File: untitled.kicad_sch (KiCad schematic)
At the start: 11 parts, among them U5 LM76005

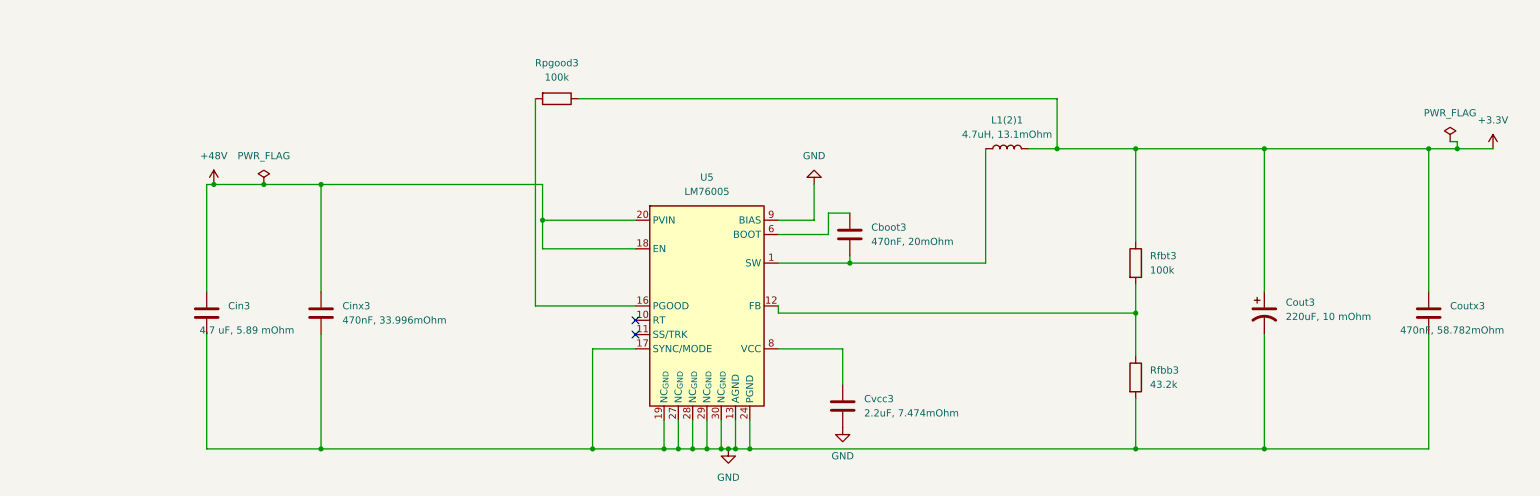
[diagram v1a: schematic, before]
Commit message: Fixed Schematics with more cost effective IC's
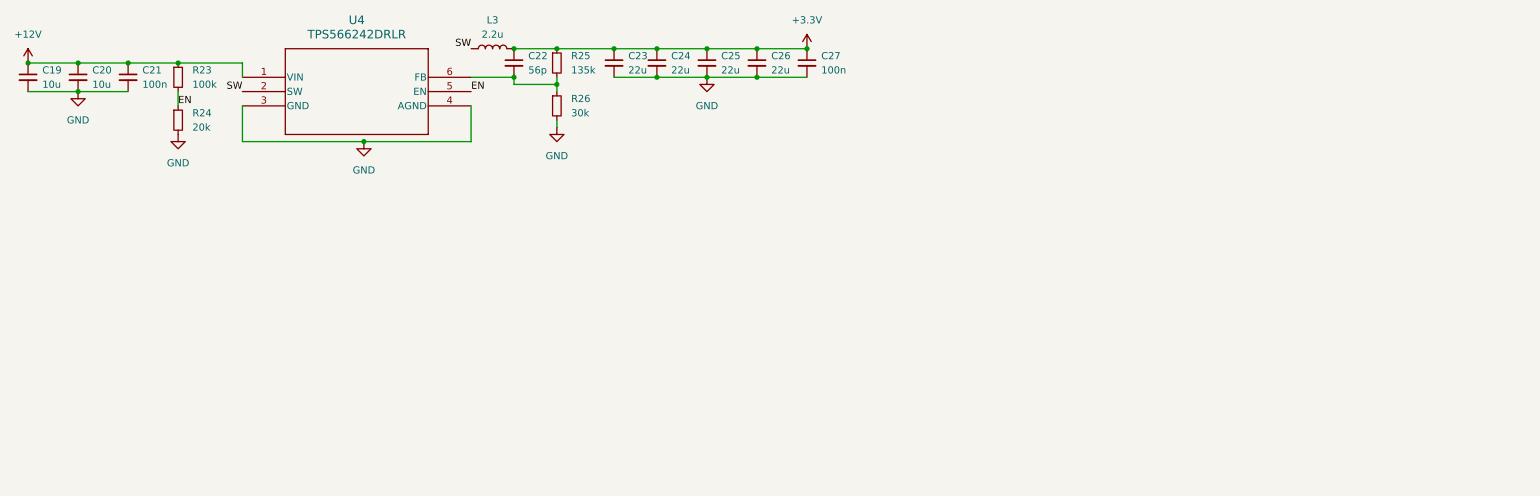
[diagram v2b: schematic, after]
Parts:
- removed Cboot3: 470nF, 20mOhm, Capacitor_SMD:C_0805_2012Metric_Pad1.18x1.45mm_HandSolder, symbol Device:C
- removed Cin3: 4.7 uF, 5.89 mOhm, symbol Device:C
- removed Cinx3: 470nF, 33.996mOhm, Capacitor_SMD:C_0805_2012Metric_Pad1.18x1.45mm_HandSolder, symbol Device:C
- removed Cout3: 220uF, 10 mOhm, Capacitor_SMD:C_0805_2012Metric_Pad1.18x1.45mm_HandSolder, symbol Device:C_Polarized_US
- removed Coutx3: 470nF, 58.782mOhm, Capacitor_SMD:C_0805_2012Metric_Pad1.18x1.45mm_HandSolder, symbol Device:C
- removed Cvcc3: 2.2uF, 7.474mOhm, Capacitor_SMD:C_0805_2012Metric_Pad1.18x1.45mm_HandSolder, symbol Device:C
- removed L1(2)1: 4.7uH, 13.1mOhm, Inductor_SMD:L_6.3x6.3_H3, symbol Device:L
- removed Rfbb3: 43.2k, Resistor_SMD:R_0201_0603Metric, symbol Device:R
- removed Rfbt3, Rpgood3: 100k, Resistor_SMD:R_0201_0603Metric, symbol Device:R
- removed U5: LM76005, Package_DFN_QFN:Texas_RNP0030B_WQFN-30-1EP_4x6mm_P0.5mm_EP1.8x4.5mm, symbol Regulator_Switching:LM76005
- added C19, C20: 10u, symbol Device:C_Small
- added C21, C27: 100n, symbol Device:C_Small
- added C22: 56p, symbol Device:C_Small
- added C23, C24, C25, C26: 22u, symbol Device:C_Small
- added L3: 2.2u, symbol Device:L
- added R23: 100k, symbol Device:R_Small
- added R24: 20k, symbol Device:R_Small
- added R25: 135k, symbol Device:R_Small
- added R26: 30k, symbol Device:R_Small
- added U4: TPS566242DRLR, footprints:SOT5x3_DRL_TEX, symbol TPS566242DRLR:TPS566242DRLR
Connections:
- net +3.3V: now also C22.1, C23.1, C24.1, C25.1, C26.1, C27.1, L3.2, R25.1
- net GND: now also C19.2, C20.2, C21.2, C23.2, C24.2, C25.2, C26.2, C27.2, R24.2, R26.2, U4.3 (GND), U4.4 (AGND)
- new net: C22.2, R25.2, R26.1, U4.6 (FB)
- new net +12V: C19.1, C20.1, C21.1, R23.1, U4.1 (VIN)
- new net EN: R23.2, R24.1, U4.5 (EN)
- new net SW: L3.1, U4.2 (SW)
- no-connect marks 2 -> 0

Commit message: feat: added footprints
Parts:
- C19, C20, C21, C22, C23, C24, C25, C26, C27, L3: footprint (none) -> Capacitor_SMD:C_0201_0603Metric_Pad0.64x0.40mm_HandSolder
- R23, R24, R25, R26: footprint (none) -> Resistor_SMD:R_0201_0603Metric_Pad0.64x0.40mm_HandSolder
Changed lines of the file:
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@@
 			)
 		)
-		(property "Footprint" ""
+		(property "Footprint" "Capacitor_SMD:C_0201_0603Metric_Pad0.64x0.40mm_HandSolder"
 			(at 100.33 33.02 0)
 			(effects
@@
 			)
 		)
-		(property "Footprint" ""
+		(property "Footprint" "Capacitor_SMD:C_0201_0603Metric_Pad0.64x0.40mm_HandSolder"
 			(at 147.32 35.56 0)
 			(effects
@@
 			)
 		)
-		(property "Footprint" ""
+		(property "Footprint" "Capacitor_SMD:C_0201_0603Metric_Pad0.64x0.40mm_HandSolder"
 			(at 26.67 38.1 0)
 			(effects
@@
 			)
 		)
-		(property "Footprint" ""
+		(property "Footprint" "Resistor_SMD:R_0201_0603Metric_Pad0.64x0.40mm_HandSolder"
 			(at 44.45 45.72 0)
 			(effects
@@
 			)
 		)
-		(property "Footprint" ""
+		(property "Footprint" "Capacitor_SMD:C_0201_0603Metric_Pad0.64x0.40mm_HandSolder"
 			(at 121.92 35.56 0)
 			(effects
@@
 			)
 		)
-		(property "Footprint" ""
+		(property "Footprint" "Resistor_SMD:R_0201_0603Metric_Pad0.64x0.40mm_HandSolder"
 			(at 44.45 38.1 0)
 			(effects
@@
 			)
 		)
-		(property "Footprint" ""
+		(property "Footprint" "Resistor_SMD:R_0201_0603Metric_Pad0.64x0.40mm_HandSolder"
 			(at 111.76 43.18 0)
 			(effects
@@
 			)
 		)
-		(property "Footprint" ""
+		(property "Footprint" "Capacitor_SMD:C_0201_0603Metric_Pad0.64x0.40mm_HandSolder"
 			(at 104.14 35.56 0)
 			(effects
@@
 			)
 		)
-		(property "Footprint" ""
+		(property "Footprint" "Capacitor_SMD:C_0201_0603Metric_Pad0.64x0.40mm_HandSolder"
 			(at 35.56 38.1 0)
 			(effects
@@
 			)
 		)
-		(property "Footprint" ""
+		(property "Footprint" "Capacitor_SMD:C_0201_0603Metric_Pad0.64x0.40mm_HandSolder"
 			(at 156.21 35.56 0)
 			(effects
@@
 			)
 		)
-		(property "Footprint" ""
+		(property "Footprint" "Capacitor_SMD:C_0201_0603Metric_Pad0.64x0.40mm_HandSolder"
 			(at 17.78 38.1 0)
 			(effects
@@
 			)
 		)
-		(property "Footprint" ""
+		(property "Footprint" "Capacitor_SMD:C_0201_0603Metric_Pad0.64x0.40mm_HandSolder"
 			(at 138.43 35.56 0)
 			(effects
@@
 			)
 		)
-		(property "Footprint" ""
+		(property "Footprint" "Resistor_SMD:R_0201_0603Metric_Pad0.64x0.40mm_HandSolder"
 			(at 111.76 35.56 0)
 			(effects
@@
 			)
 		)
-		(property "Footprint" ""
+		(property "Footprint" "Capacitor_SMD:C_0201_0603Metric_Pad0.64x0.40mm_HandSolder"
 			(at 129.54 35.56 0)
 			(effects
